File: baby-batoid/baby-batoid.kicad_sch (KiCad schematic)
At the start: 21 parts, among them J1 USB_C_Receptacle_USB2.0, U1 STM32F072CBT6, U2 PRTR5V0U2X, U3 XC6206PxxxMR-Regulator_Linear

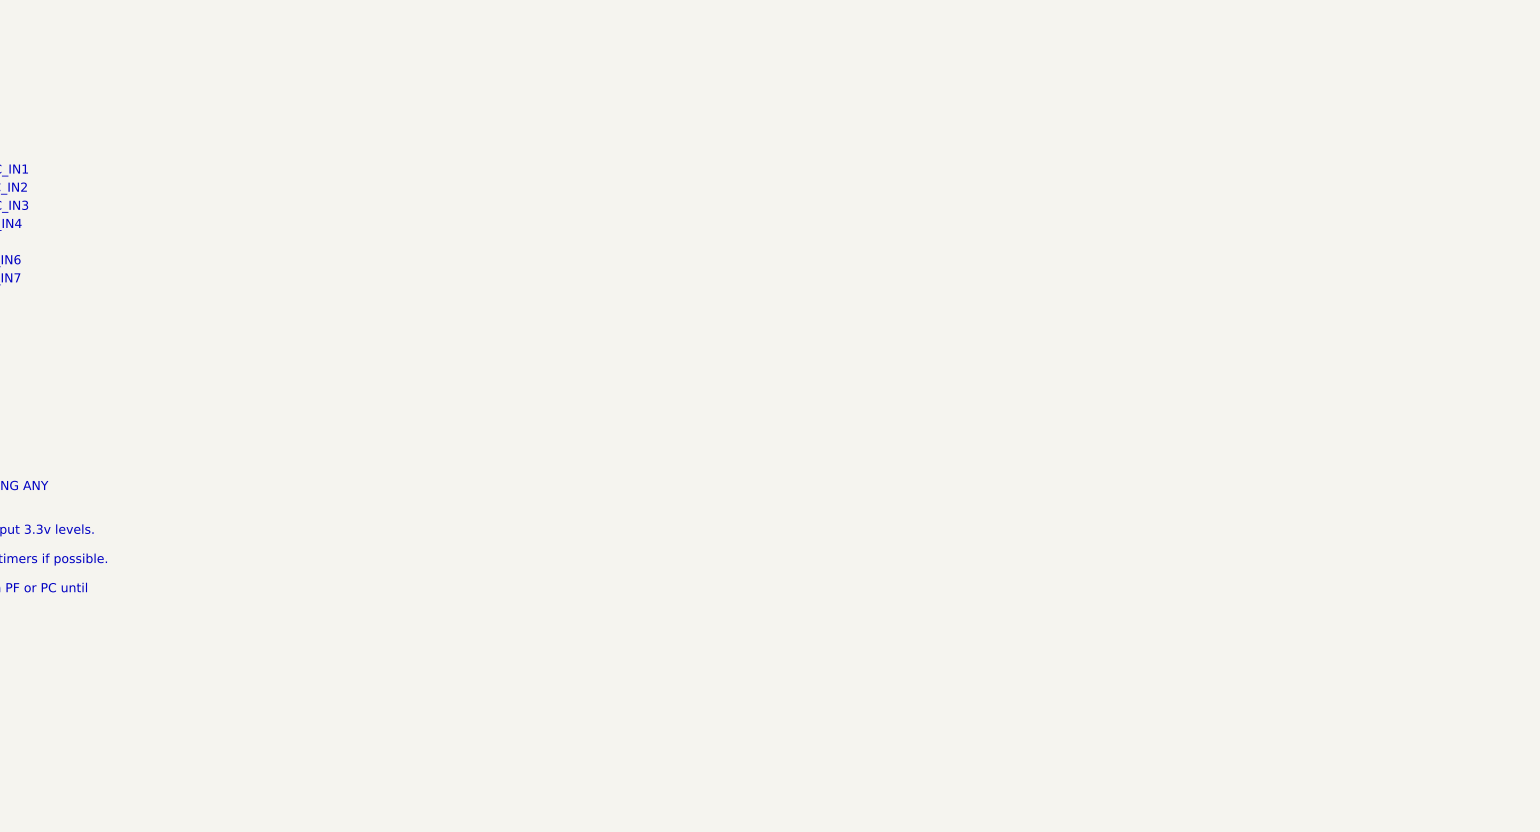
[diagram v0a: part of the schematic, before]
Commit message: built baby batoid :D
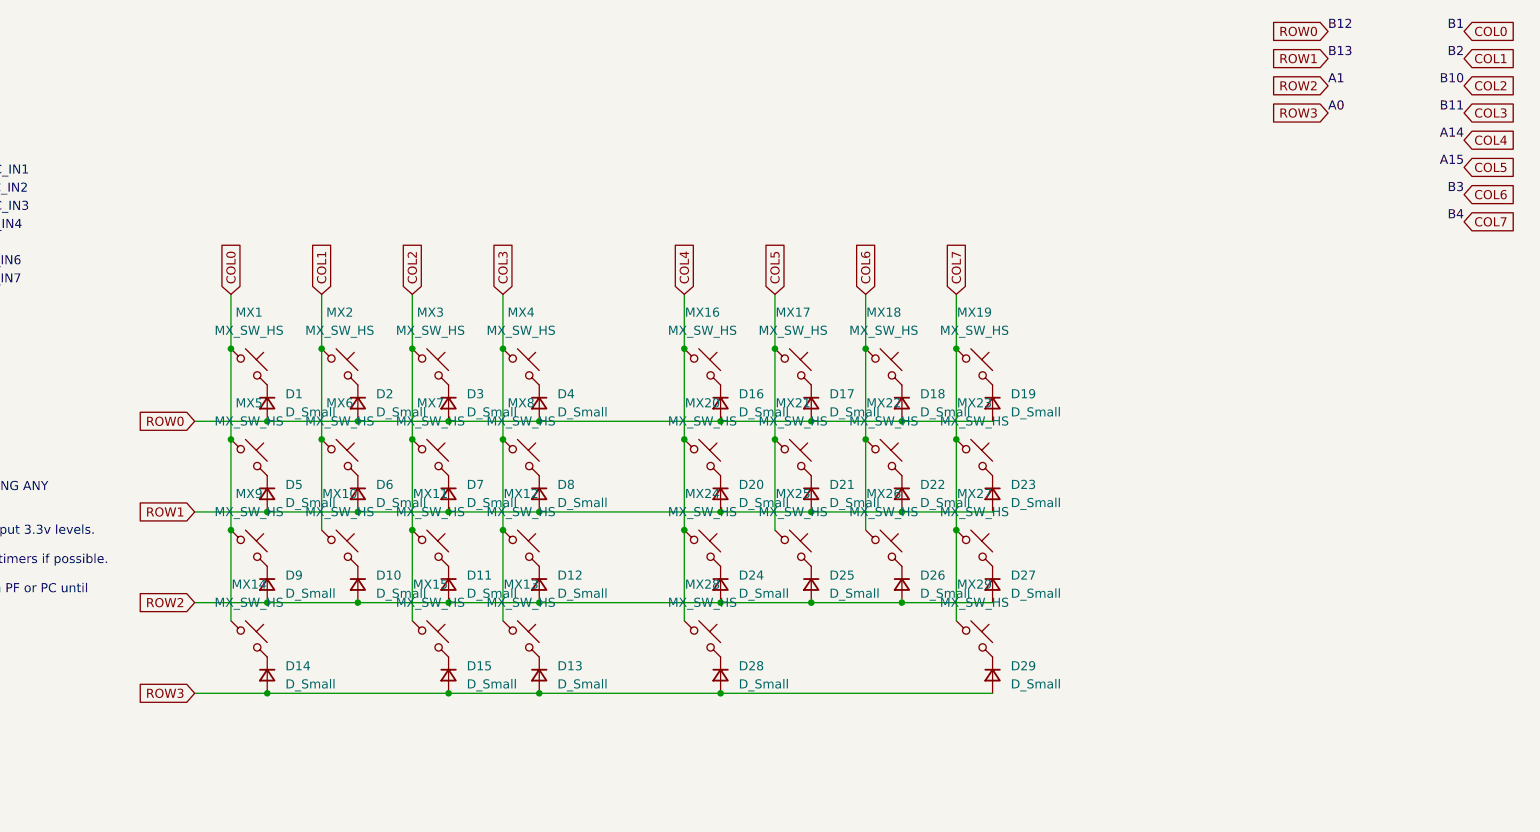
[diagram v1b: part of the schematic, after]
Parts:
- added D1, D10, D11, D12, D13, D14, D15, D16, D17, D18, D19, D2, D20, D21, D22, D23, D24, D25, D26, D27, D28, D29, D3, D4, D5, D6, D7, D8, D9: D_Small, Diode_SMD:D_SOD-123, symbol Device:D_Small
- added MX1, MX10, MX11, MX12, MX13, MX14, MX15, MX16, MX17, MX18, MX19, MX2, MX20, MX21, MX22, MX23, MX24, MX25, MX26, MX27, MX28, MX29, MX3, MX4, MX5, MX6, MX7, MX8, MX9: MX_SW_HS, marbastlib-mx:SW_MX_HS_CPG151101S11_1u, symbol marbastlib-mx:MX_SW_HS_CPG151101S11
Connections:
- net A0 renamed ROW3
- net ROW3: now also D13.2 (A), D14.2 (A), D15.2 (A), D28.2 (A), D29.2 (A)
- net A1 renamed ROW2
- net ROW2: now also D10.2 (A), D11.2 (A), D12.2 (A), D24.2 (A), D25.2 (A), D26.2 (A), D27.2 (A), D9.2 (A)
- net A14 renamed COL4
- net COL4: now also MX16.1, MX20.1, MX24.1, MX28.1
- net A15 renamed COL5
- net COL5: now also MX17.1, MX21.1, MX25.1
- net B1 renamed COL0
- net COL0: now also MX1.1, MX14.1, MX5.1, MX9.1
- net B10 renamed COL2
- net COL2: now also MX11.1, MX15.1, MX3.1, MX7.1
- net B11 renamed COL3
- net COL3: now also MX12.1, MX13.1, MX4.1, MX8.1
- net B12 renamed ROW0
- net ROW0: now also D1.2 (A), D16.2 (A), D17.2 (A), D18.2 (A), D19.2 (A), D2.2 (A), D3.2 (A), D4.2 (A)
- net B13 renamed ROW1
- net ROW1: now also D20.2 (A), D21.2 (A), D22.2 (A), D23.2 (A), D5.2 (A), D6.2 (A), D7.2 (A), D8.2 (A)
- net B2 renamed COL1
- net COL1: now also MX10.1, MX2.1, MX6.1
- net B3 renamed COL6
- net COL6: now also MX18.1, MX22.1, MX26.1
- net B4 renamed COL7
- net COL7: now also MX19.1, MX23.1, MX27.1, MX29.1
- new net: D16.1 (K), MX16.2
- new net: D15.1 (K), MX15.2
- new net: D19.1 (K), MX19.2
- new net: D21.1 (K), MX21.2
- new net: D17.1 (K), MX17.2
- new net: D1.1 (K), MX1.2
- new net: D4.1 (K), MX4.2
- new net: D5.1 (K), MX5.2
- new net: D28.1 (K), MX28.2
- new net: D18.1 (K), MX18.2
- new net: D3.1 (K), MX3.2
- new net: D8.1 (K), MX8.2
- new net: D25.1 (K), MX25.2
- new net: D24.1 (K), MX24.2
- new net: D27.1 (K), MX27.2
- new net: D13.1 (K), MX13.2
- new net: D20.1 (K), MX20.2
- new net: D29.1 (K), MX29.2
- new net: D2.1 (K), MX2.2
- new net: D22.1 (K), MX22.2
- new net: D23.1 (K), MX23.2
- new net: D14.1 (K), MX14.2
- new net: D12.1 (K), MX12.2
- new net: D7.1 (K), MX7.2
- new net: D6.1 (K), MX6.2
- new net: D10.1 (K), MX10.2
- new net: D26.1 (K), MX26.2
- new net: D11.1 (K), MX11.2
- new net: D9.1 (K), MX9.2
